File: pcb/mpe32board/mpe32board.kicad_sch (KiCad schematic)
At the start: 38 parts, among them J1 Conn_ST_STDC14, J2 USB_C_Receptacle_USB2.0_16P, J46 Conn_02x10_Counter_Clockwise, SW1 SW_Push, SW2 SW_Push, U10 W9812G6KH-75, U2 USBLC6-2P6, U3 AMS1117-3.3, U9 STM32H743IITx

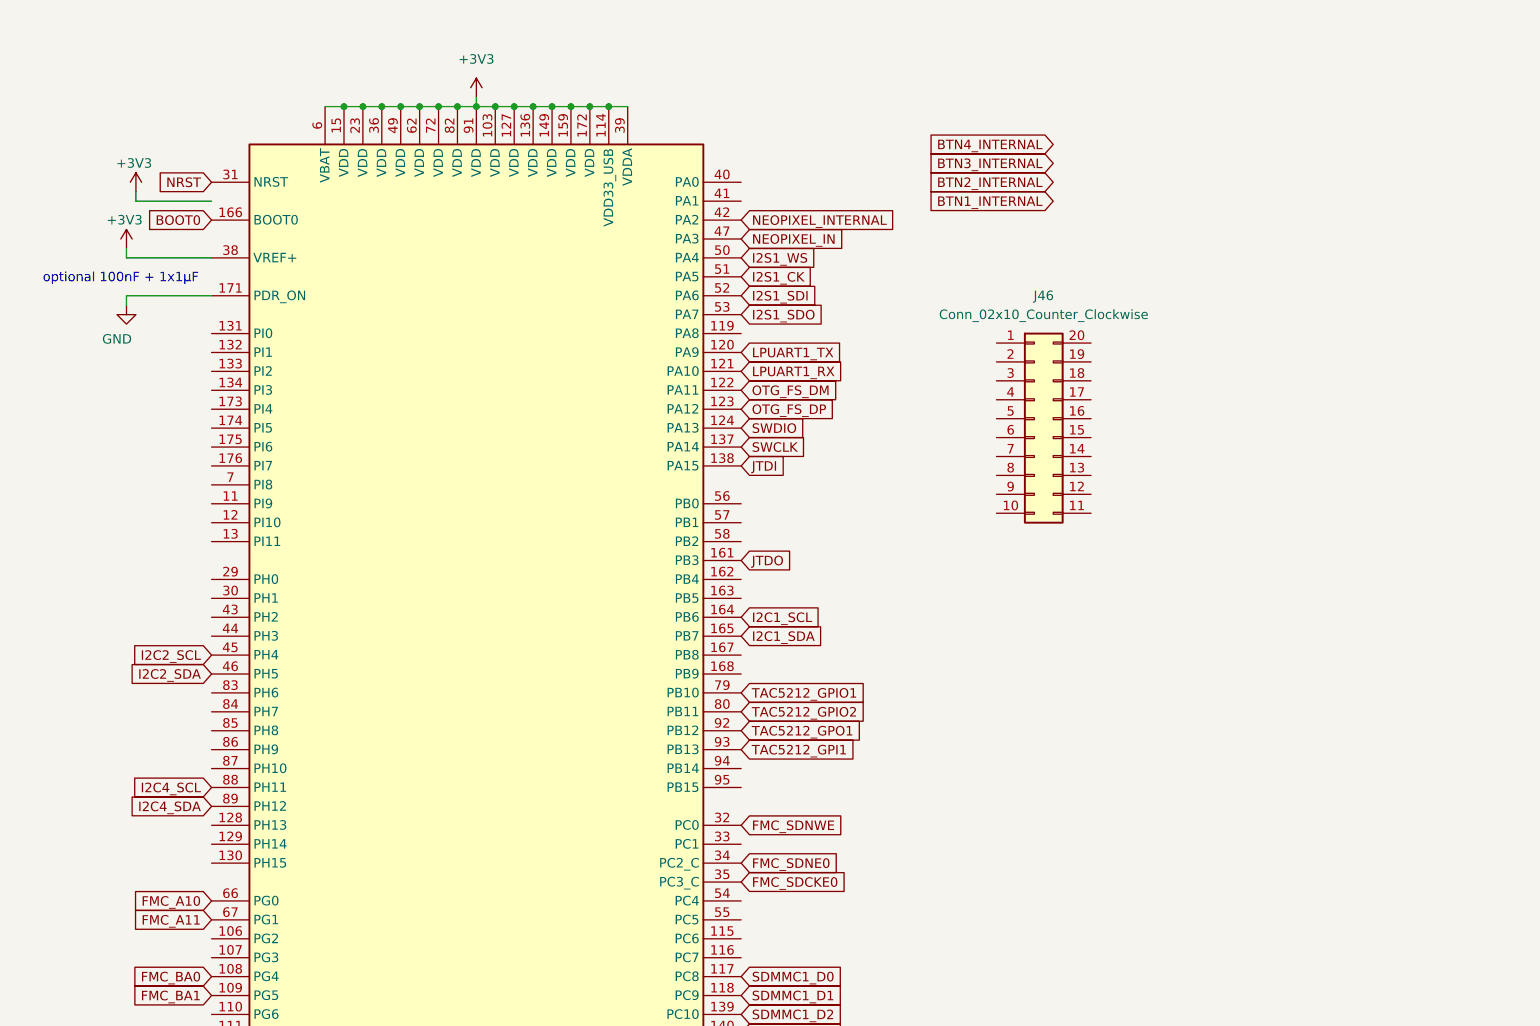
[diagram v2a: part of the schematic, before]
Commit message: board layout stuff
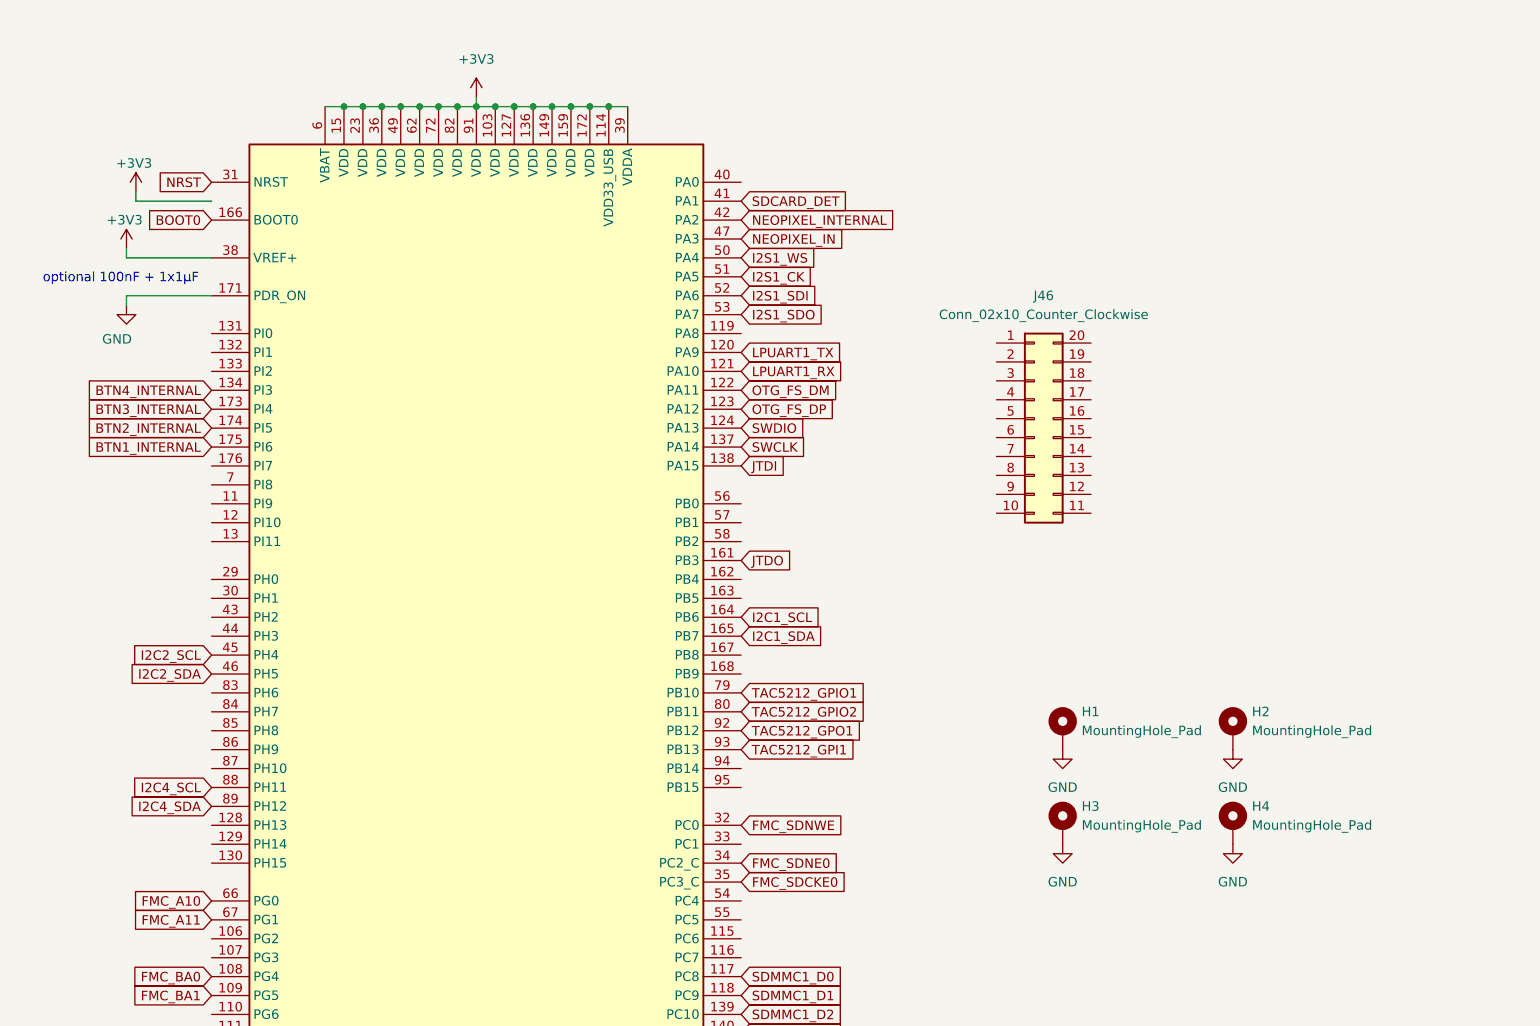
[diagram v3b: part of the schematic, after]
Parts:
- added H1, H2, H3, H4: MountingHole_Pad, MountingHole:MountingHole_3.2mm_M3_DIN965_Pad, symbol Mechanical:MountingHole_Pad
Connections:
- net BTN1_INTERNAL: now also U9.175 (PI6)
- net BTN2_INTERNAL: now also U9.174 (PI5)
- net BTN3_INTERNAL: now also U9.173 (PI4)
- net BTN4_INTERNAL: now also U9.134 (PI3)
- net GND: now also H1.1, H2.1, H3.1, H4.1
- net SDCARD_DET: now reaches U9.41 (PA1)
